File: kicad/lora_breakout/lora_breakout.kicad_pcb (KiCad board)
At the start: 2 copper layers, 27.9 x 20.3 mm, 3 parts, among them J1 Conn_01x08, J2 Conn_01x08, U1 RFM95W-915S2

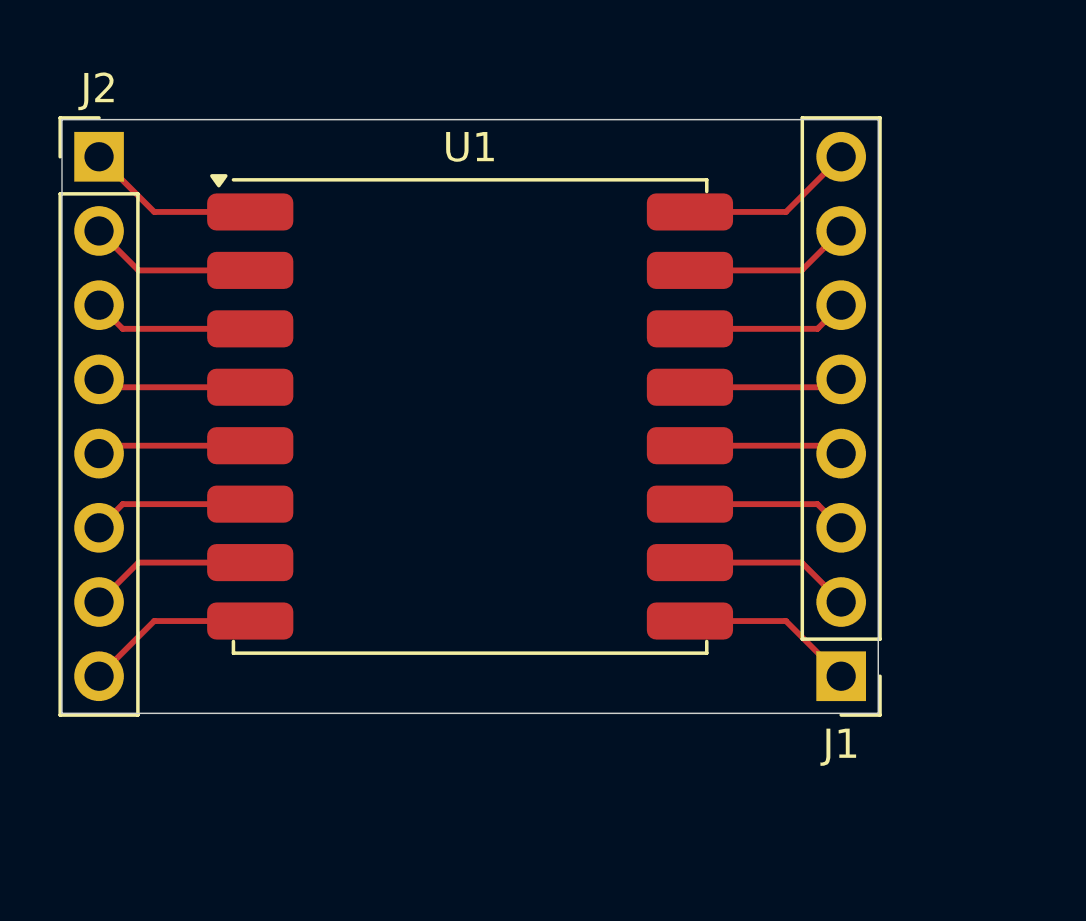
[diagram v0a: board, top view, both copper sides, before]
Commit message: updated lora breakout
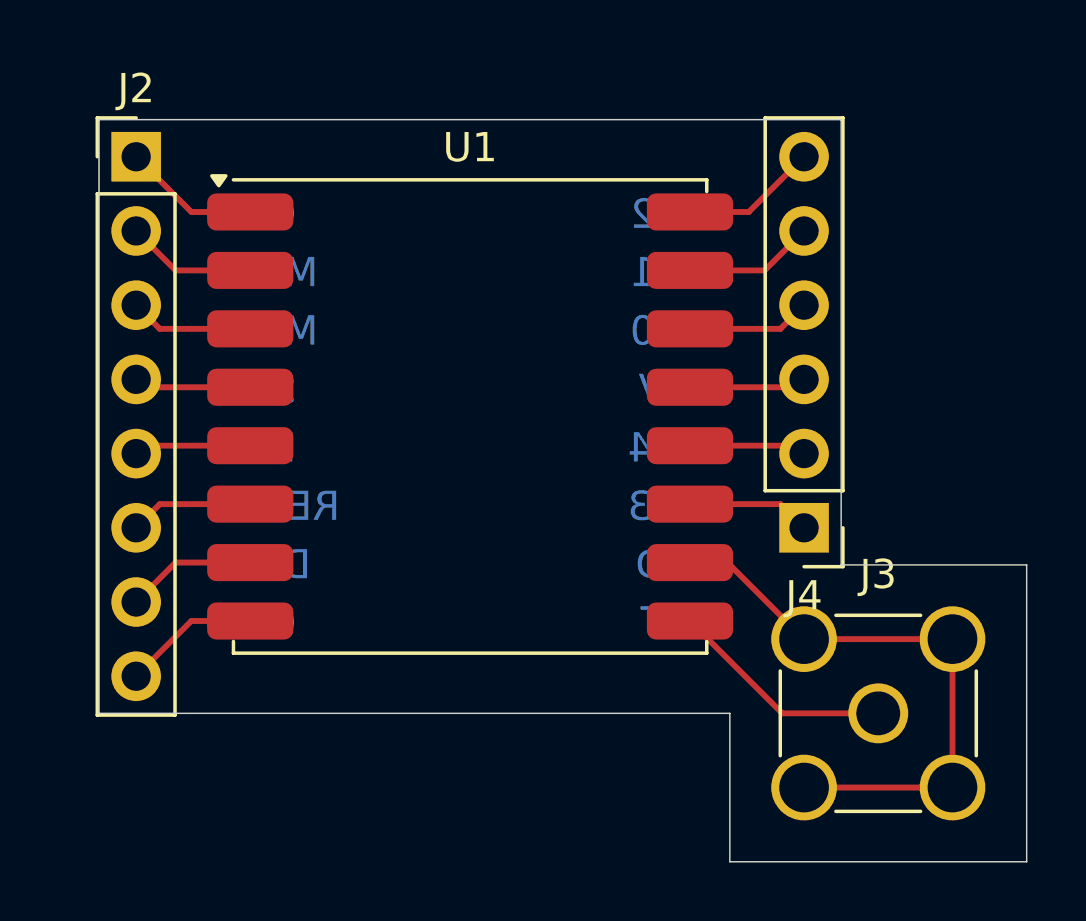
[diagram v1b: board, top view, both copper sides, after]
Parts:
- removed J1: Conn_01x08, Connector_PinHeader_2.54mm:PinHeader_1x08_P2.54mm_Vertical
- added J3: Conn_Coaxial, Connector_Coaxial:SMA_Amphenol_901-144_Vertical, F.Cu at (153.7, 95.2)
- added J4: Conn_01x06, Connector_PinHeader_2.54mm:PinHeader_1x06_P2.54mm_Vertical, F.Cu at (151.1, 88.9)
- moved J2 1.27 mm to (128.3, 76.2)
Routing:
- net Net-(J3-Ext): track 5.73 -> 20.2 mm
- net Net-(J3-In): track 5.96 -> 7.75 mm
- net Net-(J4-Pin_5): track 5.73 -> 4.46 mm
- net Net-(J4-Pin_4): track 5.51 -> 4.24 mm
- net Net-(J4-Pin_1): track 5.51 -> 4.24 mm
- net Net-(J2-Pin_8): track 5.96 -> 4.69 mm
- net Net-(J2-Pin_7): track 5.73 -> 4.46 mm
- net Net-(J2-Pin_6): track 5.51 -> 4.24 mm
- net Net-(J2-Pin_3): track 5.51 -> 4.24 mm
- net Net-(J2-Pin_2): track 5.73 -> 4.46 mm
- net Net-(J2-Pin_1): track 5.96 -> 4.69 mm
- net Net-(J2-Pin_4): track 5.29 -> 4.02 mm
- net Net-(J2-Pin_5): track 5.67 -> 4.40 mm
- net Net-(J4-Pin_3): track 5.29 -> 4.02 mm
- net Net-(J4-Pin_2): track 5.29 -> 4.02 mm
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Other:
- board size 27.9 x 20.3 mm -> 31.8 x 25.4 mm
- board text added: "3.3V"
- board text added: "ANT"
- board text added: "DIO0"
- board text added: "DIO1"
- board text added: "DIO2"
- board text added: "DIO3"
- board text added: "DIO4"
- board text added: "DIO5"
- board text added: "GND"
- board text added: "MISO"
- board text added: "MOSI"
- board text added: "NSS"
- board text added: "RESET"
- board text added: "SCK"
